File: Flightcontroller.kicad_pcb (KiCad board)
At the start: 4 copper layers, 78.9 x 65.2 mm, 74 parts, among them J2 JST?, J3 Conn_01x03_Socket, J4 Conn_01x03_Socket, J5 Conn_01x03_Socket, J6 XT60, J7 Conn_01x04_Socket, J8 Conn_01x04_Socket, J9 Conn_01x04_Socket, P2 USB_C_Plug_USB2.0, SW1 SW_SPST, SW2 SW_DIP_x02, U2 ALED8102S, U3 lm3940 LDO, U5 STM32F103C8Tx, U6 BMP280 (Barometer), U7 MPU-6050 (IMU), U8 NEO-M9N, Y2 abracon abm3 8mhz

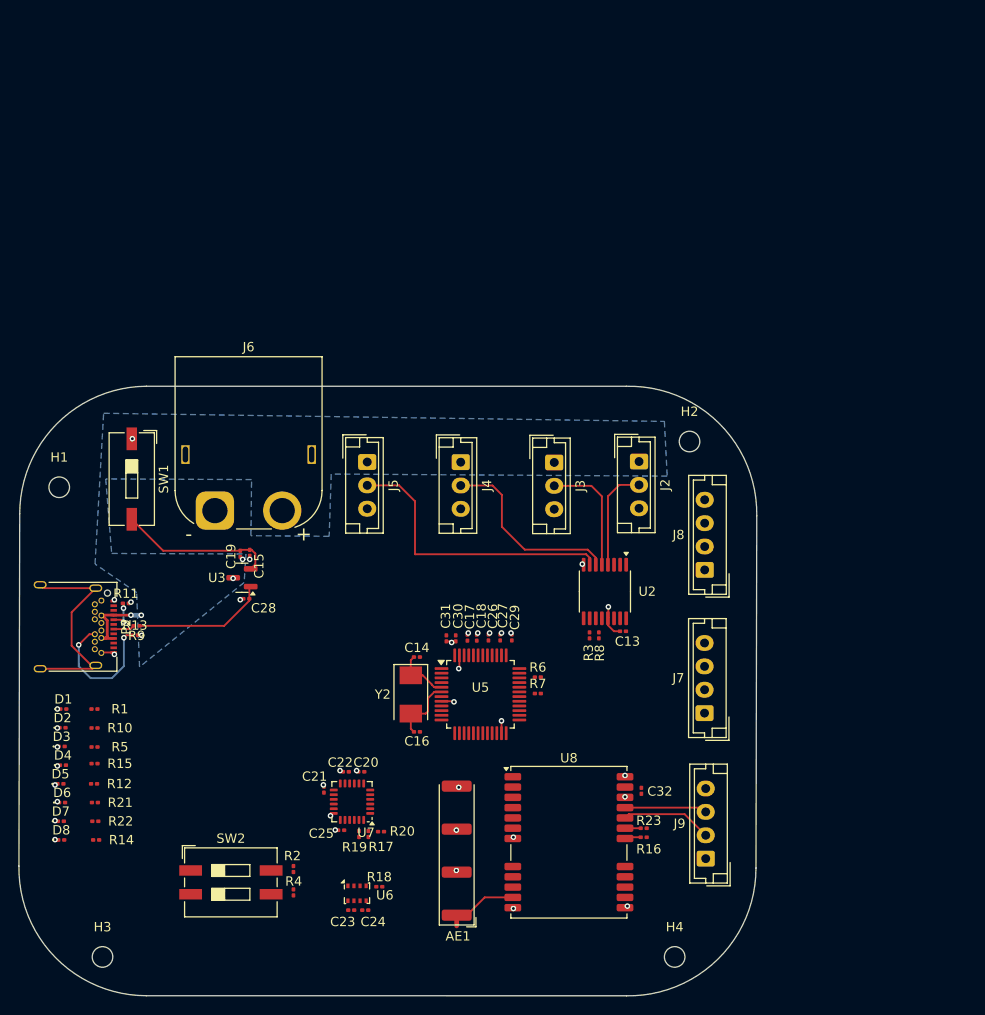
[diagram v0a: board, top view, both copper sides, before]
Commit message: Add files via upload
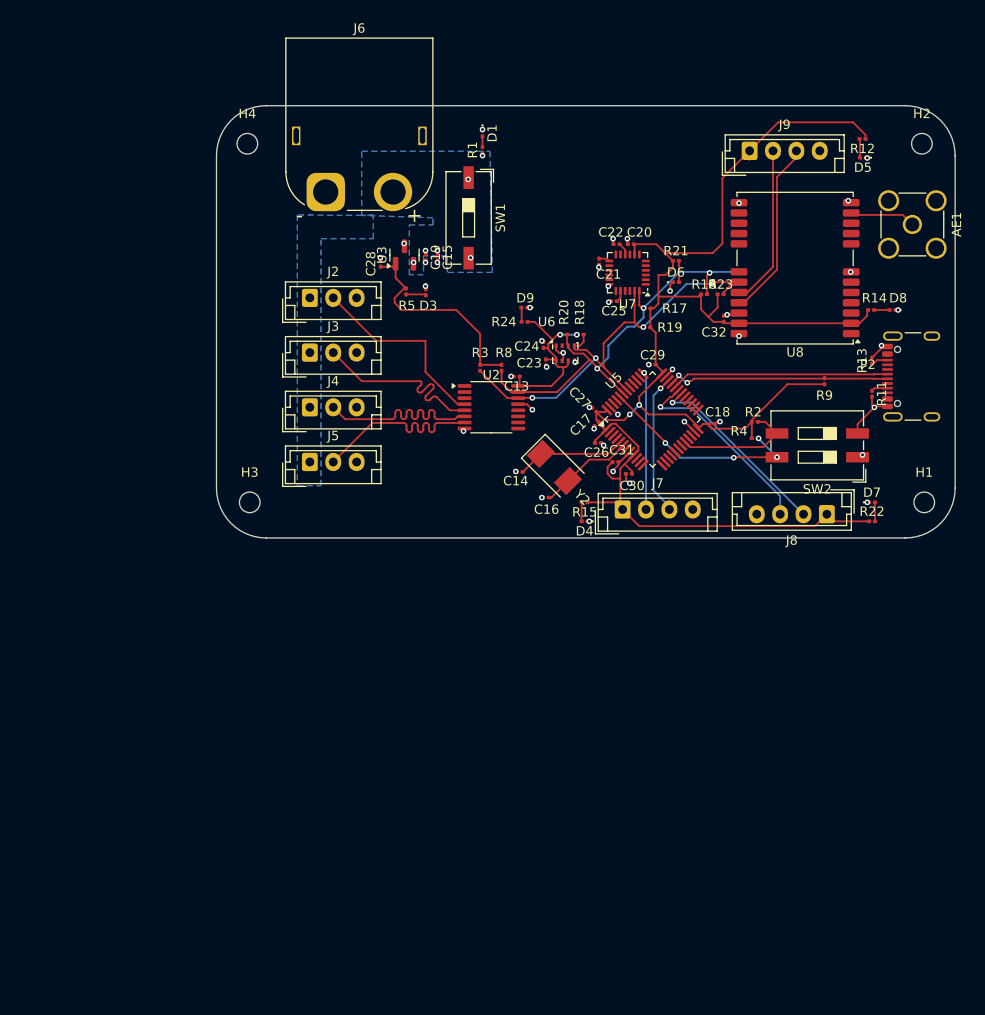
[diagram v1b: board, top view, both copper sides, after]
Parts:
- removed D2: USB_LED, LED_SMD:LED_0201_0603Metric
- removed R10: 500 , 0603, Resistor_SMD:R_0201_0603Metric
- removed R6, R7: 20, Resistor_SMD:R_0201_0603Metric
- added D9: BAR_LED, LED_SMD:LED_0201_0603Metric, F.Cu at (199.3, 69.1)
- added R24: 220 , 0603, Resistor_SMD:R_0201_0603Metric, F.Cu at (199.3, 70.6)
- AE1: footprint RF_Antenna:Antenova_SR4G013_GPS -> Connector_Coaxial:SMA_Amphenol_132134-11_Vertical
- P2: footprint Connector_USB:USB_C_Receptacle_Amphenol_12401548E4-2A -> Connector_USB:USB_C_Receptacle_GCT_USB4105-xx-A_16P_TopMnt_Horizontal
- R1: value 220 , 0603 -> 560 , 0603
- R2, R4: value 10k 0603 -> 4.7k 0603
- R9: value 4.7k,0603 -> 1.5k,0603
- moved D5 108.9 mm to (235.5, 53.1), turned to 180 degrees
- moved R12 107.3 mm to (235.5, 51.1)
- moved D8 105.4 mm to (238.7, 69.3), turned to 180 degrees
- moved R14 100.4 mm to (236.4, 69.3), turned to 0 degrees
- moved H4 98.2 mm to (169.7, 51.6)
- moved P2 95.3 mm to (241.8, 76.5), turned to 90 degrees
- moved D7 93.2 mm to (236.5, 89.9)
- moved H1 92.5 mm to (242.1, 89.9)
- moved R22 89.0 mm to (236.5, 91.9), turned to 0 degrees
- moved D6 86.1 mm to (215.5, 66.4)
- moved R21 85.0 mm to (215.5, 64.1), turned to 0 degrees
- moved R13 84.1 mm to (236.5, 74.8), turned to 90 degrees
- moved R11 82.9 mm to (236.5, 78.3), turned to -90 degrees
- moved AE1 82.8 mm to (240.8, 60.2), turned to -90 degrees
- moved SW2 78.2 mm to (230.6, 83.8), turned to 180 degrees
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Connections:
- C15 pad 1: Net-(SW1-B) -> +5V
- C17 pad 1: Net-(C17-Pad1) -> +3.3V
- C18 pad 1: Net-(C17-Pad1) -> +3.3V
- C19 pad 1: Net-(SW1-B) -> +5V
- C26 pad 1: Net-(C17-Pad1) -> +3.3V
- C27 pad 1: Net-(C17-Pad1) -> +3.3V
- C29 pad 1: Net-(C17-Pad1) -> +3.3V
- C30 pad 1: Net-(C30-Pad1) -> +3.3V
- C31 pad 1: Net-(C30-Pad1) -> +3.3V
- P2 pad A4: +5V -> unconnected-(P2-VBUS-PadA4)
- P2 pad A6: Net-(P2-D+) -> USBDP
- P2 pad A7: Net-(P2-D-) -> USBDN
- P2 pad A9: +5V -> unconnected-(P2-VBUS-PadA4)
- P2 pad B4: +5V -> unconnected-(P2-VBUS-PadA4)
- P2 pad B9: +5V -> unconnected-(P2-VBUS-PadA4)
- R2 pad 1: Net-(R2-Pad1) -> +3.3V
- R4 pad 1: Net-(R4-Pad1) -> BOOT1
- R4 pad 2: BOOT1 -> +3.3V
- R9 pad 2: Net-(P2-D-) -> USBDP
- SW1 pad 2: Net-(SW1-B) -> +5V
- SW2 pad 1: +3.3V -> GND
- SW2 pad 2: +3.3V -> GND
- SW2 pad 3: Net-(R4-Pad1) -> BOOT1
- SW2 pad 4: Net-(R2-Pad1) -> BOOT0
- U3 pad 2: Net-(SW1-B) -> +5V
- U5 pad 32: USBDM -> USBDN
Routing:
- net +3.3V: track 14.4 -> 216.7 mm, vias 0 -> 4
- net I2C1_SCL: track 1.68 -> 51.7 mm, vias 0 -> 4
- net I2C1_SDA: track 1.74 -> 48.2 mm, vias 0 -> 3
- net USBDP: track 0.00 -> 23.5 mm, vias 0 -> 2
- net unconnected-(P2-SHIELD-PadS1): track 22.9 -> 0.00 mm
- net USBDN: track 0.00 -> 22.7 mm
- net BOOT0: track 0.00 -> 22.5 mm, vias 0 -> 4
- net USART1_RX: track 0.00 -> 21.7 mm, vias 0 -> 1
- net USART1_TX: track 0.00 -> 20.9 mm, vias 0 -> 1
- net Net-(SW1-B): track 16.7 -> 0.00 mm
- net JTMS/SWDIO: track 0.00 -> 15.2 mm, vias 0 -> 1
- net JTCK/SWCLK: track 0.00 -> 15.0 mm, vias 0 -> 1
- net GND: track 10.1 -> 24.2 mm, vias 40 -> 44
- net BOOT1: track 0.00 -> 13.2 mm
- net Net-(P2-VCONN): track 14.4 -> 1.81 mm, vias 2 -> 0
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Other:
- board size 78.9 x 65.2 mm -> 79 x 46.2 mm
